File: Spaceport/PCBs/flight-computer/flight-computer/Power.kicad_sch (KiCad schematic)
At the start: 26 parts, among them IC1 AP7362-33SP-13, IC2 AP7362-33SP-13, J10 5.0VOUT, J9 3.3VOUT, U6 TPS62A03DRLR

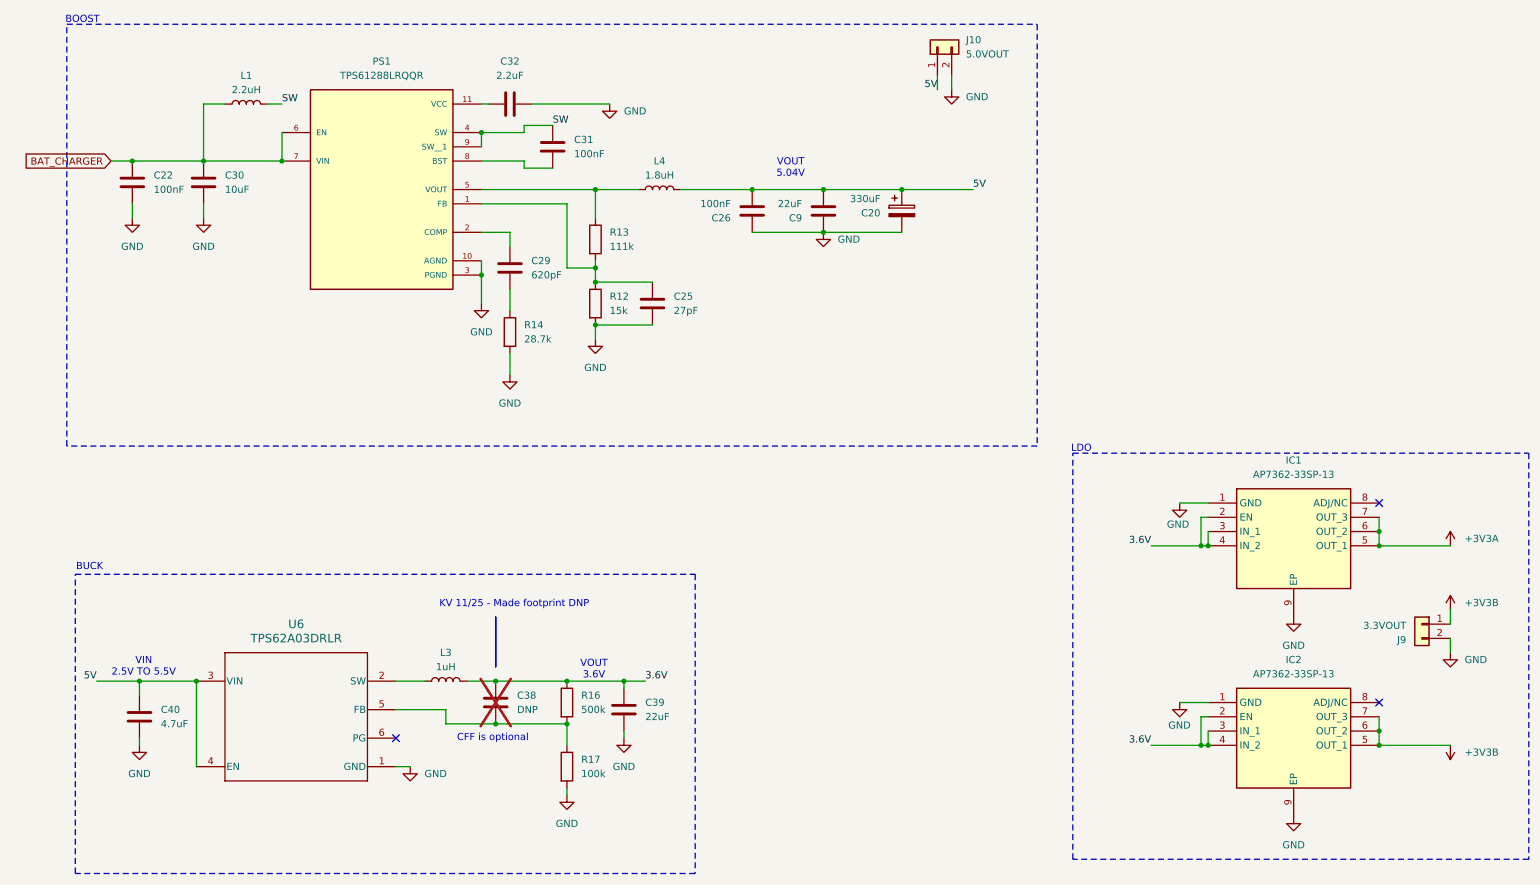
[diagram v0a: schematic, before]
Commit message: Revert "Merge branch 'main' of https://github.com/Terrapin-Rocket-Team/SRAD-Avionics"
This reverts commit e5f68e4e525f2a5ad7eebbc917cc2807b67ca5e1, reversing
changes made to 8a40e2e341d8980ca528983581171a8bd9cc0146.
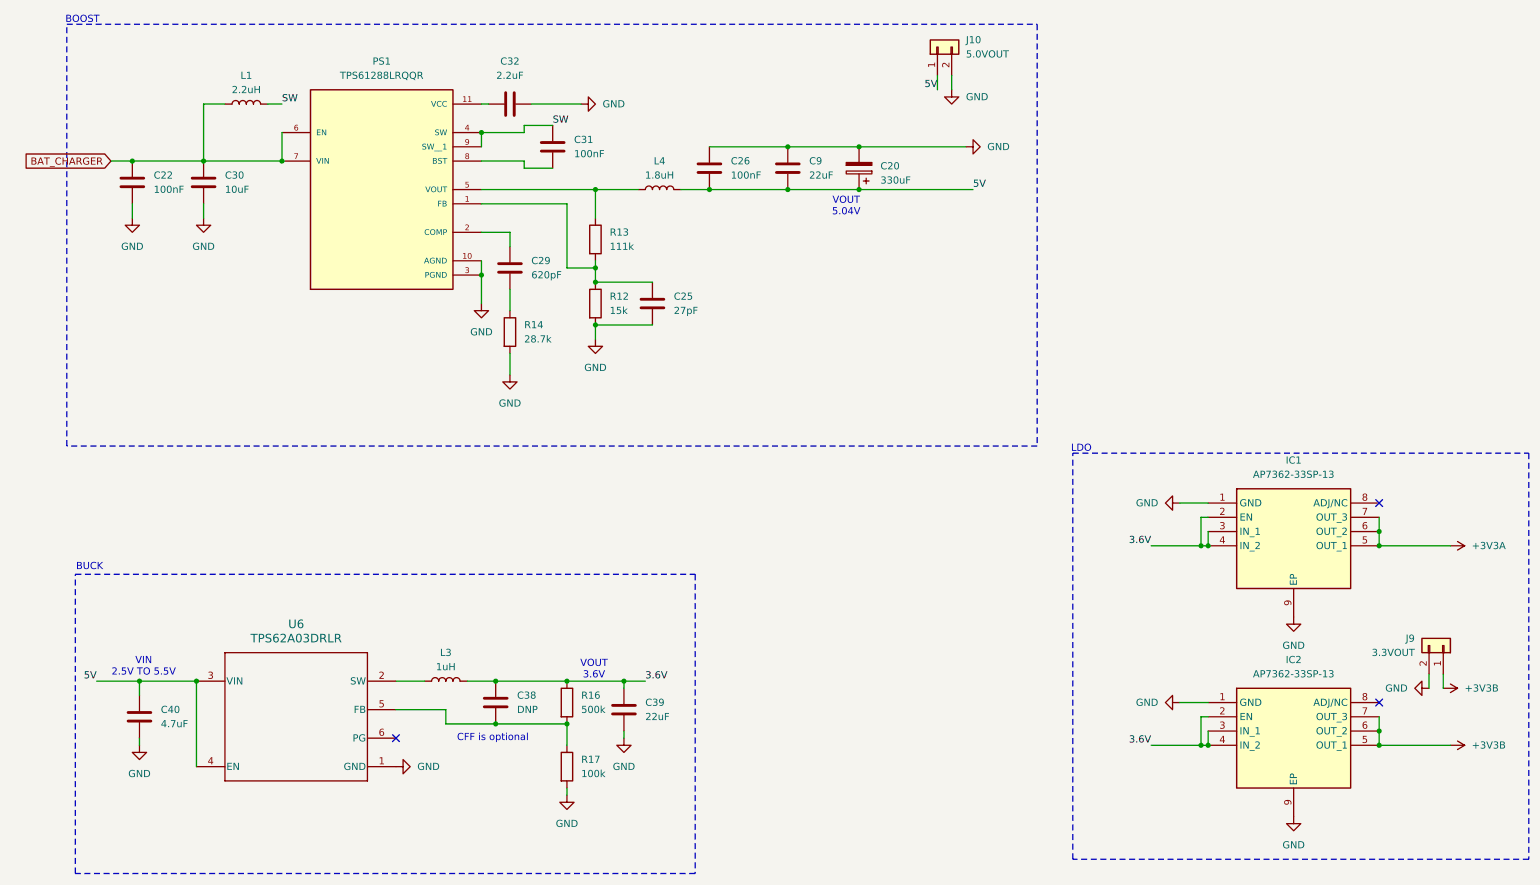
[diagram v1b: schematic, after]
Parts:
- C20: footprint Capacitor_SMD:CP_Elec_10x10 -> (none)
- C22, C25, C26, C29, C30, C31, C32, C39, C40, C9: footprint Capacitor_SMD:C_0603_1608Metric_Pad1.08x0.95mm_HandSolder -> (none)
- C38: now fitted
- IC1, IC2: footprint Package_SO:Diodes_SO-8EP -> SOIC127P600X150-9N
- J10, J9: footprint Connector_JST:JST_XH_B2B-XH-A_1x02_P2.50mm_Vertical -> (none)
- L1, L3, L4: footprint Inductor_SMD:L_0805_2012Metric_Pad1.05x1.20mm_HandSolder -> (none)
- PS1: footprint Package_DFN_QFN:Texas_VQFN-HR-20_3x2.5mm_P0.5mm_RQQ0011A -> TPS61288LRQQR:CONV_TPS61288LRQQR
- R12, R13, R14, R16, R17: footprint Resistor_SMD:R_0603_1608Metric_Pad0.98x0.95mm_HandSolder -> (none)
- U6: footprint Package_TO_SOT_SMD:SOT-563 -> DRL0006A-MFG
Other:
- note removed: "KV 11/25 - Made footprint DNP"
- moved on the sheet: C20, C26, C9, J9

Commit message: Restore flight computer files
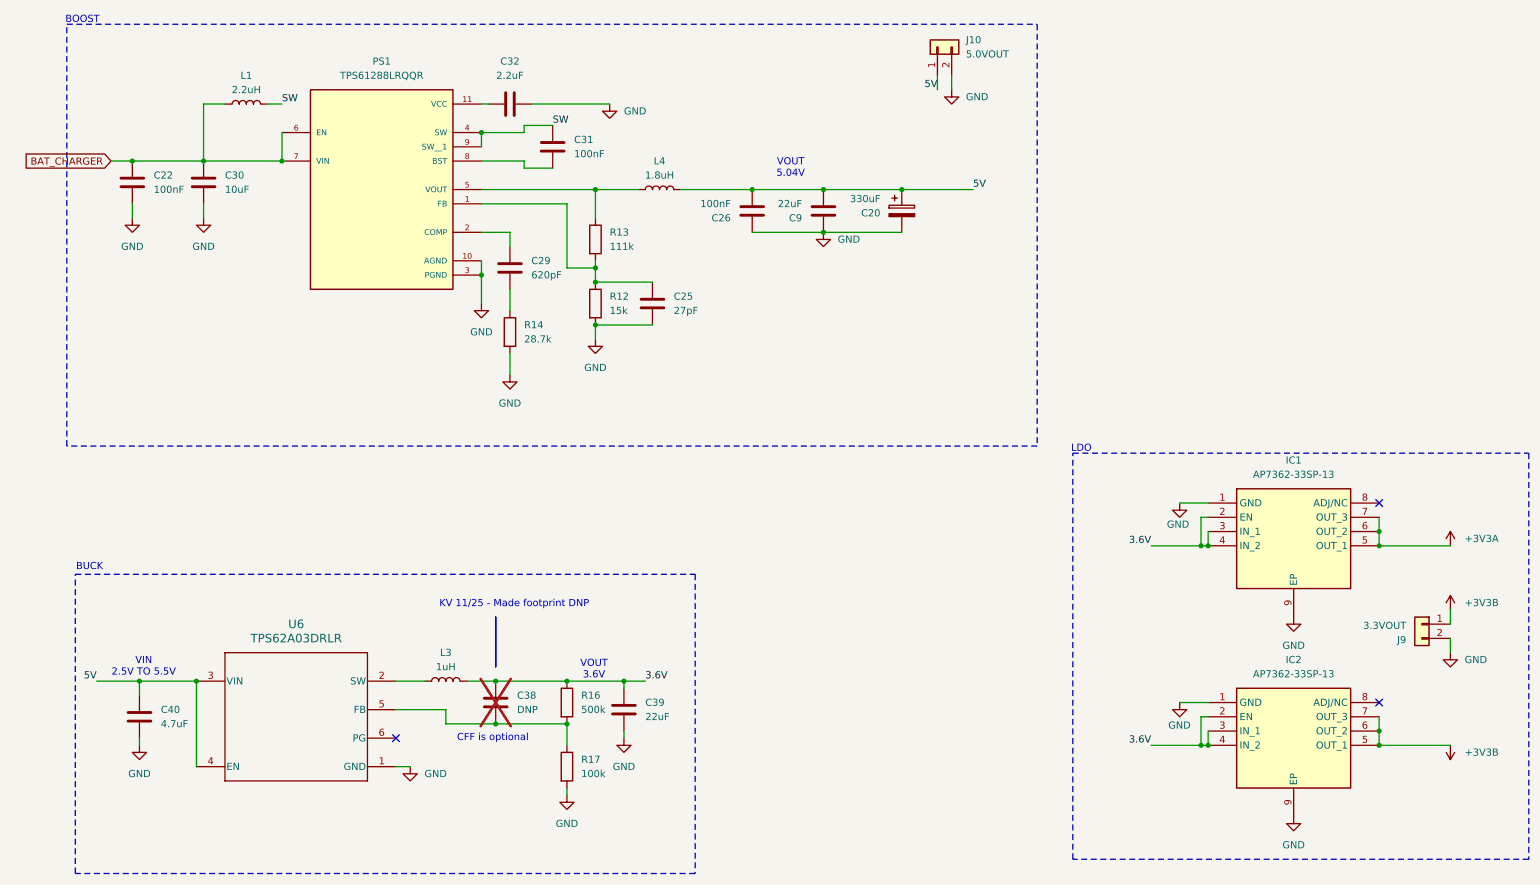
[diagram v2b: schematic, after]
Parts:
- C20: footprint (none) -> Capacitor_SMD:CP_Elec_10x10
- C22, C25, C26, C29, C30, C31, C32, C39, C40, C9: footprint (none) -> Capacitor_SMD:C_0603_1608Metric_Pad1.08x0.95mm_HandSolder
- C38: now not fitted
- IC1, IC2: footprint SOIC127P600X150-9N -> Package_SO:Diodes_SO-8EP
- J10, J9: footprint (none) -> Connector_JST:JST_XH_B2B-XH-A_1x02_P2.50mm_Vertical
- L1, L3, L4: footprint (none) -> Inductor_SMD:L_0805_2012Metric_Pad1.05x1.20mm_HandSolder
- PS1: footprint TPS61288LRQQR:CONV_TPS61288LRQQR -> Package_DFN_QFN:Texas_VQFN-HR-20_3x2.5mm_P0.5mm_RQQ0011A
- R12, R13, R14, R16, R17: footprint (none) -> Resistor_SMD:R_0603_1608Metric_Pad0.98x0.95mm_HandSolder
- U6: footprint DRL0006A-MFG -> Package_TO_SOT_SMD:SOT-563
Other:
- note added: "KV 11/25 - Made footprint DNP"
- moved on the sheet: C20, C26, C9, J9
